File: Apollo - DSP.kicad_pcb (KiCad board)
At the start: 4 copper layers, 74.9 x 58 mm, 80 parts, among them J1 USB_C_Receptacle_USB2.0, J2 Conn_01x04, J3 Conn_01x04, J4 MEM2067-02-180-00-A_REVB, J5 Conn_01x06, J6 Conn_01x04, U1 NCP115ASN330T2G, U3 USBLC6-2SC6, U4 STM32F401RBTx, U5 23K256, U6 MCP4725xxx-xCH, U7 MCP602, U8 MCP602, Y1 16MHz

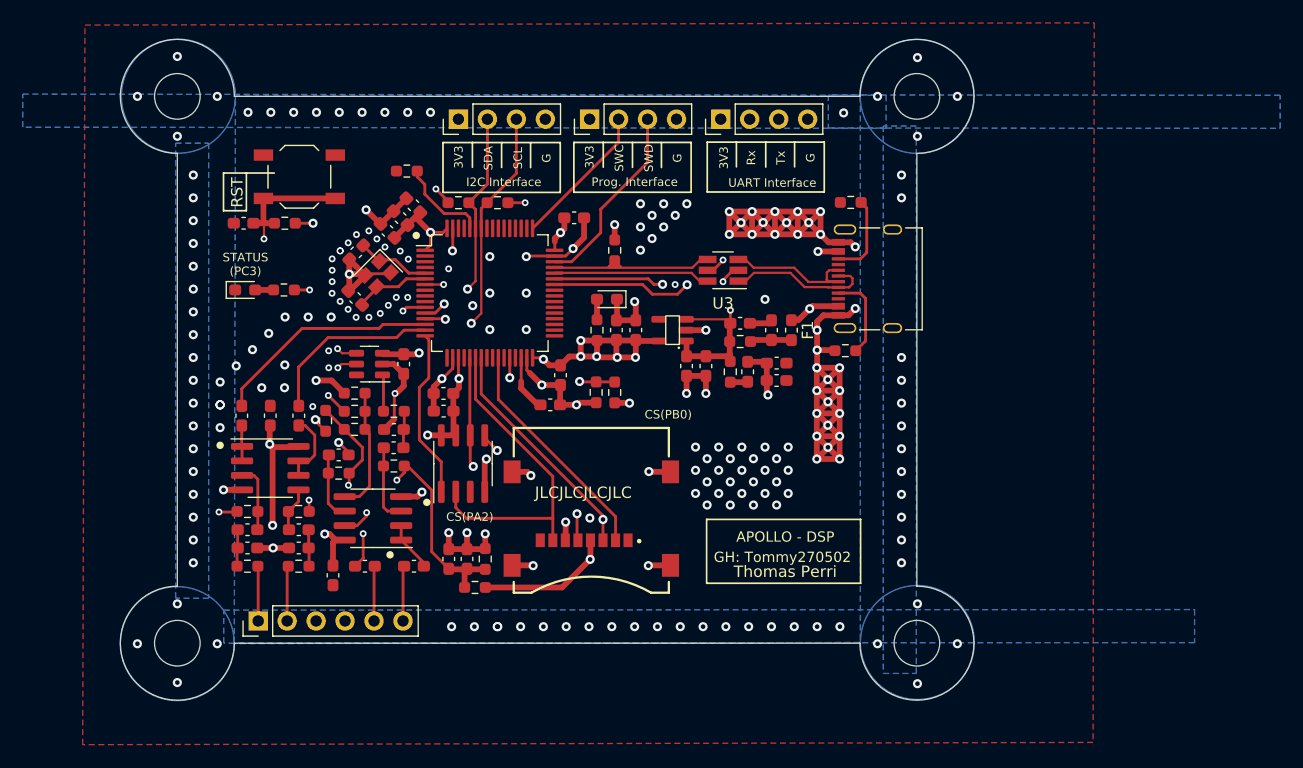
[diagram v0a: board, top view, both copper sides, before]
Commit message: refreshing design
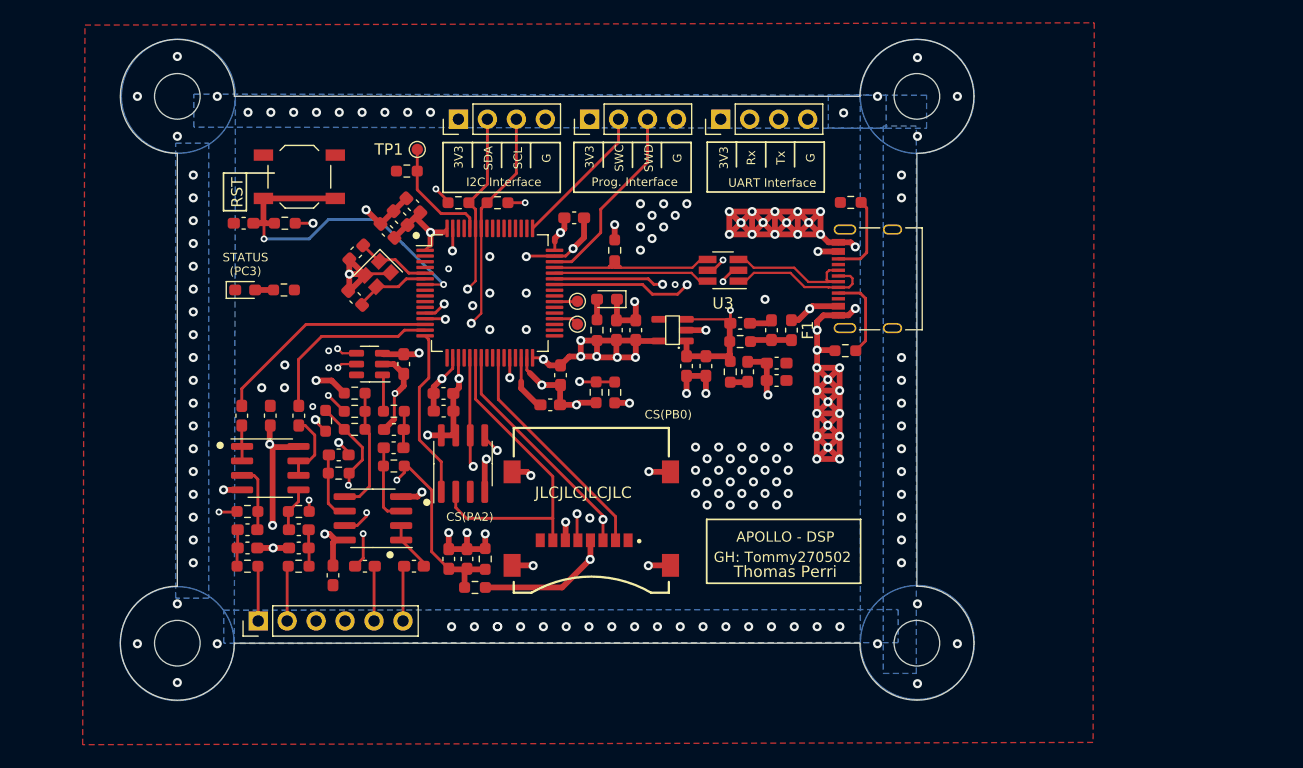
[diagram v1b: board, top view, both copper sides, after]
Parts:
- added TP1: TestPoint, TestPoint:TestPoint_Pad_D1.0mm, F.Cu at (120.9, 66.4)
- added TP2: TestPoint, TestPoint:TestPoint_Pad_D1.0mm, F.Cu at (134.9, 79.7)
- added TP3: TestPoint, TestPoint:TestPoint_Pad_D1.0mm, F.Cu at (134.9, 81.7)
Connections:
- U4 pad 36: unconnected-(U4-PB15-Pad36) -> Net-(U4-PB15)
- U4 pad 39: unconnected-(U4-PC8-Pad39) -> Net-(U4-PC8)
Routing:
- net Net-(U4-PC3): track 14.7 -> 0.00 mm, vias 2 -> 0
- net Net-(U4-PB15): track 0.00 -> 2.20 mm
- net BOOT0: track 8.03 -> 10.1 mm
- net Net-(U4-PC8): track 0.00 -> 2.02 mm
- net GND: vias 220 -> 188
